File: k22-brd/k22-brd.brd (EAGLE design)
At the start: 21.6 x 63.5 mm, 35 parts, among them J1 61302011121, J2 61302011121, J3 CORTEX_DEBUG_PTH

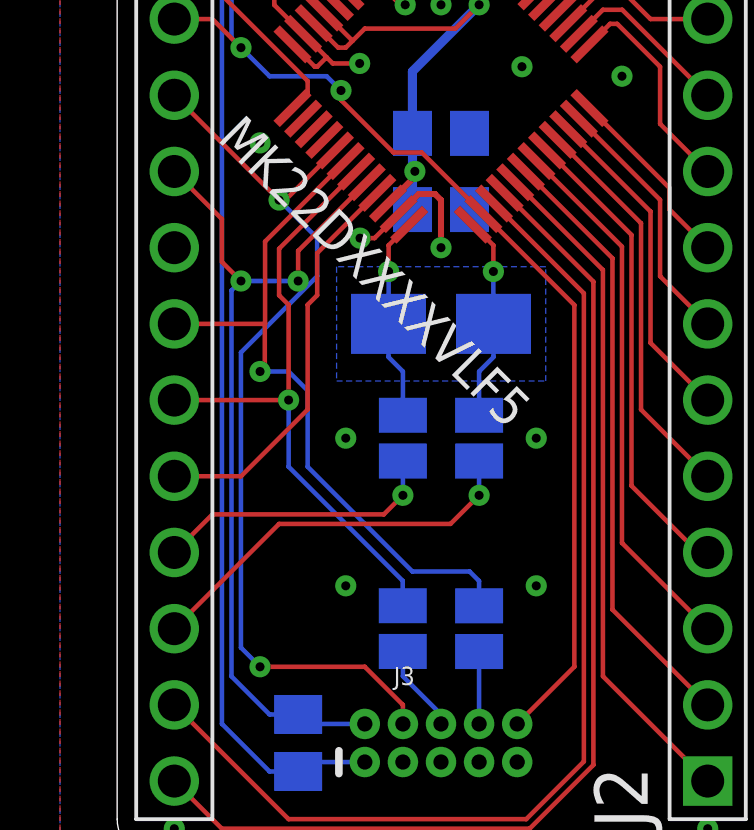
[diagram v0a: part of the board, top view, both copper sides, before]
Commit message: Prvni verze shieldu
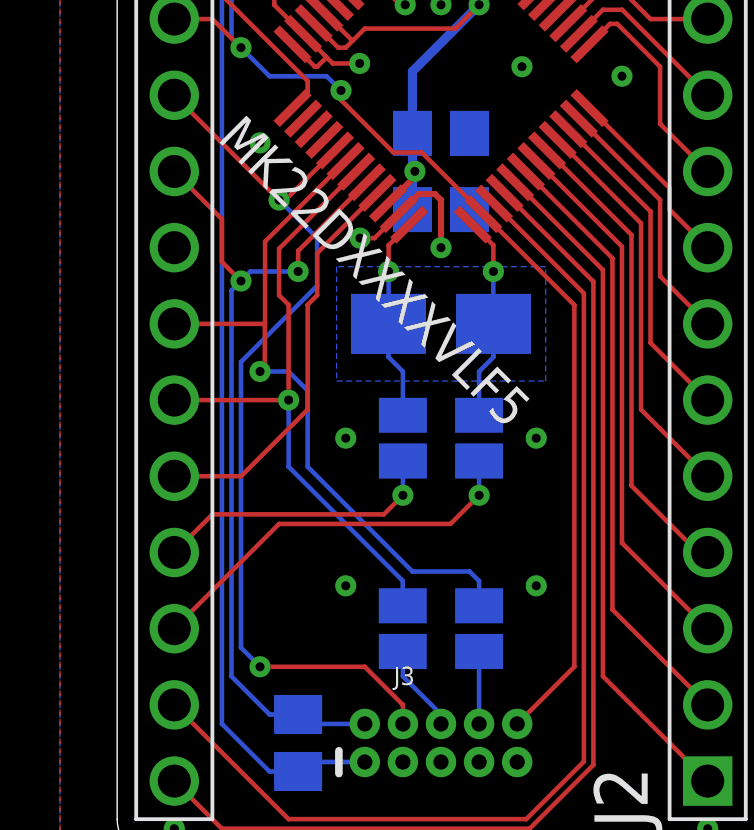
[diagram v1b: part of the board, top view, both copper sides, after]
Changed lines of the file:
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@@
 <setting verticaltext="up"/>
 </settings>
-<grid distance="25" unitdist="mil" unit="mil" style="dots" multiple="1" display="yes" altdistance="6.25" altunitdist="mil" altunit="mil"/>
+<grid distance="12.5" unitdist="mil" unit="mil" style="dots" multiple="1" display="yes" altdistance="6.25" altunitdist="mil" altunit="mil"/>
 <layers>
 <layer number="1" name="Top" color="4" fill="1" visible="yes" active="yes"/>
@@
 <contactref element="J3" pad="4"/>
 <contactref element="J1" pad="11"/>
-<wire x1="4.1275" y1="16.8275" x2="6.6675" y2="19.3675" width="0.1524" layer="16"/>
-<wire x1="4.1275" y1="6.985" x2="4.1275" y2="16.8275" width="0.1524" layer="16"/>
-<wire x1="6.6675" y1="19.3675" x2="6.6675" y2="20.6375" width="0.1524" layer="16"/>
+<wire x1="4.1275" y1="16.51" x2="6.6675" y2="19.05" width="0.1524" layer="16"/>
+<wire x1="4.1275" y1="6.985" x2="4.1275" y2="16.51" width="0.1524" layer="16"/>
+<wire x1="6.6675" y1="19.05" x2="6.6675" y2="20.6375" width="0.1524" layer="16"/>
 <wire x1="6.6675" y1="20.6375" x2="5.3975" y2="21.9075" width="0.1524" layer="16"/>
 <via x="5.3975" y="21.9075" extent="1-16" drill="0.3"/>
@@
 <contactref element="J3" pad="2"/>
 <contactref element="RS2" pad="2"/>
-<wire x1="8.320125" y1="22.499465625" x2="6.032446875" y2="20.2117875" width="0.1524" layer="1"/>
-<wire x1="6.032446875" y1="20.2117875" x2="6.0325" y2="19.20875" width="0.1524" layer="1"/>
+<wire x1="8.320125" y1="22.499465625" x2="6.0324625" y2="20.211803125" width="0.1524" layer="1"/>
+<wire x1="6.0324625" y1="20.211803125" x2="6.0325" y2="19.52625" width="0.1524" layer="1"/>
 <contactref element="J1" pad="12"/>
-<via x="6.0325" y="19.20875" extent="1-16" drill="0.3"/>
-<wire x1="6.0325" y1="19.20875" x2="4.1275" y2="19.20875" width="0.1524" layer="16"/>
+<via x="6.0325" y="19.52625" extent="1-16" drill="0.3"/>
+<wire x1="6.0325" y1="19.52625" x2="4.445" y2="19.52625" width="0.1524" layer="16"/>
+<wire x1="4.445" y1="19.52625" x2="4.1275" y2="19.20875" width="0.1524" layer="16"/>
 <via x="4.1275" y="19.20875" extent="1-16" drill="0.3"/>
 <wire x1="4.1275" y1="19.20875" x2="3.4925" y2="19.84375" width="0.1524" layer="1"/>
